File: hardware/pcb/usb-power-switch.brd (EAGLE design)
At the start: 50.8 x 27.9 mm, 15 parts, among them IC1 TPS2024, IC2 LD1117V33

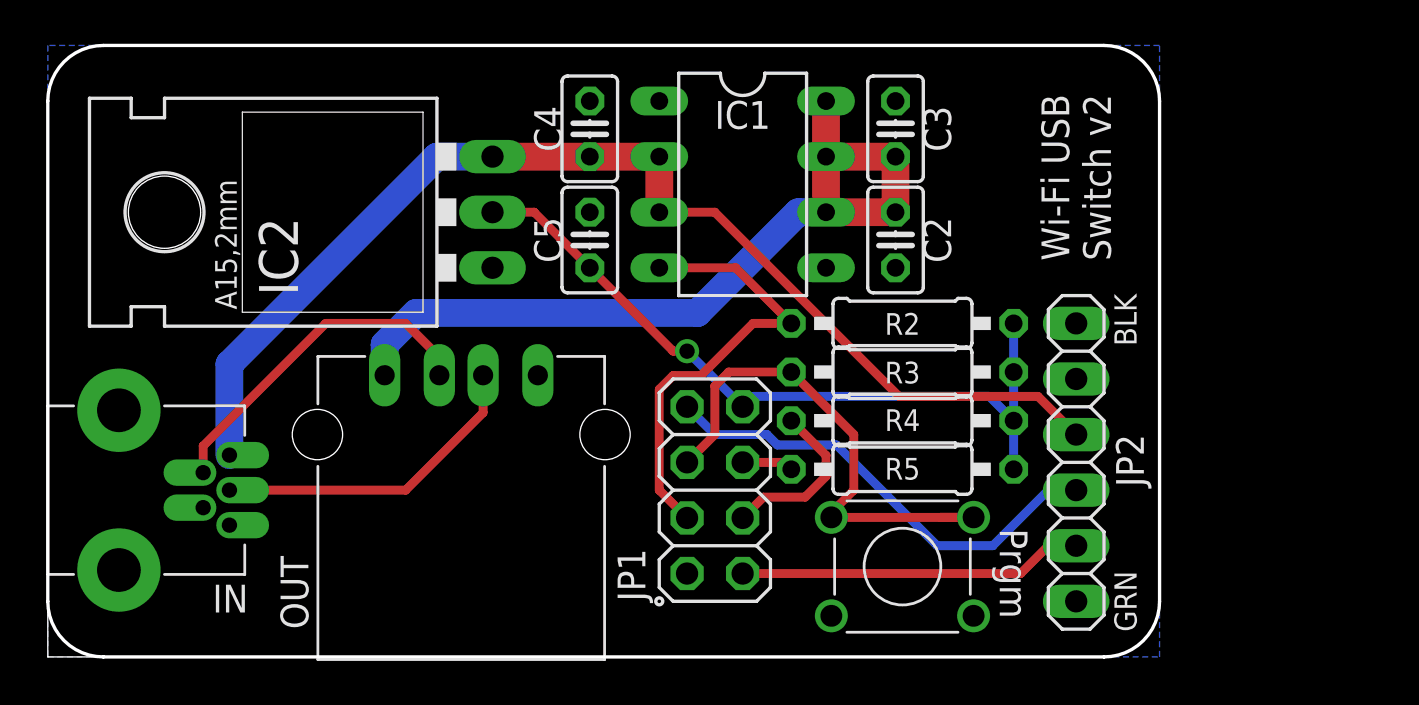
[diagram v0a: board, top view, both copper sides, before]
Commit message: Updated PCB to v3
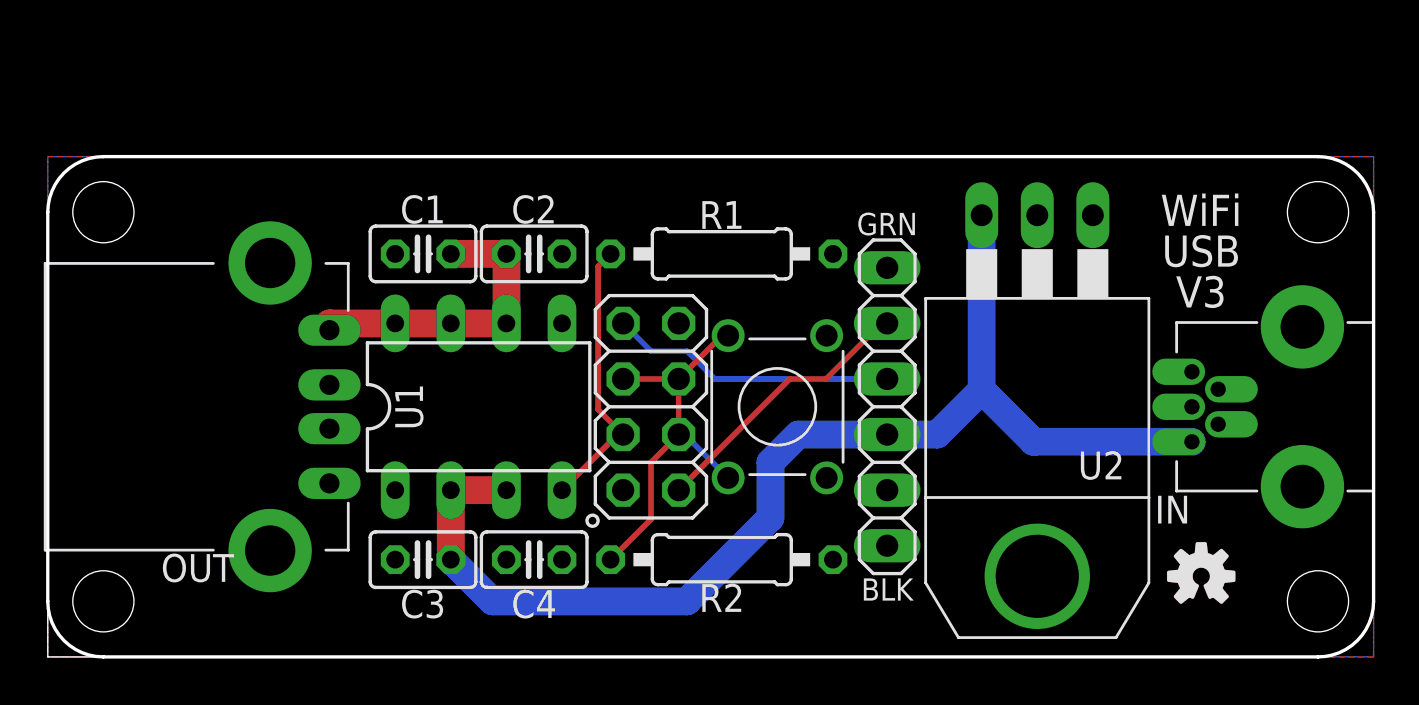
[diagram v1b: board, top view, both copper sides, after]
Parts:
- removed C5: 10uF, rcl:C025-025X050
- removed IC1: TPS2024, ic-package:DIL08
- removed IC2: LD1117V33, SparkFun-PowerIC:78XXL
- removed JP1: ESP-01, pinhead:2X04
- removed JP2: FTDI 3.3V, pinhead:1X06
- removed R3, R4, R5: 10K, rcl:0207/10
- added C1: 22uF, rcl:C025-025X050
- added J1: ESP8266-01, pinhead:2X04
- added J2: FTDI 3.3V, pinhead:1X06
- added R1: 10K, rcl:0207/10
- added U$1: (no value), SparkFun-Aesthetics:OSHW-LOGO-S
- added U$2: (no value), SparkFun-Aesthetics:OSHW-LOGO-S_COPPER
- added U1: TPS2024, ic-package:DIL08
- added U2: LD1117V33, my-custom:TO-220
- C3: value 22uF -> 0.1uF
- C4: value 0.1uF -> 10uF
- IN: value USB-MINI-B -> WM17115-ND
- OUT: value USB-A -> UE27AC54100-ND
- S1: value TACTILE-BUTTON-MJTP1230 -> MJTP1230
- moved IN 57.5 mm to (57.4, 11.4), turned to 90 degrees
- moved C3 29.2 mm to (17.1, 4.45), turned to 180 degrees
- moved C4 19.8 mm to (22.2, 4.45), turned to 180 degrees
- moved C2 16.5 mm to (22.2, 18.4), turned to 0 degrees
- moved R2 13.6 mm to (30.8, 4.45)
- moved S1 9.27 mm to (33.3, 11.4), turned to 90 degrees
- moved OUT 8.82 mm to (10.2, 11.4), turned to 270 degrees
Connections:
- removed net CH_PD: JP1.3, R4.1
- removed net D+: IN.D+, OUT.P$3
- removed net D-: IN.D-, OUT.P$2
- removed net GPIO0: JP1.6, R3.1, S1.P$1, S1.P$3
- removed net RST: JP1.5, R5.1
- new net PU: J1.3, J1.5, J1.6, R2.1, S1.P$1, S1.P$3
- net /EN: now also J1.4, R1.1, U1.4; no longer IC1.4, JP1.4, R2.1
- net DTR: now also J2.6; no longer JP2.6
- net GND: now also C1.2, IN.GND1, IN.GND4, J1.2, J2.1, J2.2, OUT.P$5, OUT.P$6, U1.1, U2.P$1; no longer C3.2, C5.2, IC1.1, IC2.IN, JP1.2, JP2.1, JP2.2
- net RXI: now also J1.8, J2.4; no longer JP1.8, JP2.4
- net TXO: now also J1.1, J2.5; no longer JP1.1, JP2.5
- net VCC: now also C4.1, J1.7, R1.2, U2.P$2, U2.P$4; no longer C5.1, IC2.GND, JP1.7, R3.2, R4.2, R5.2
- net VIN: now also C3.1, J2.3, U1.2, U1.3, U2.P$3; no longer C4.1, IC1.2, IC1.3, IC2.OUT, JP2.3
- net VOUT: now also C1.1, U1.6, U1.7, U1.8; no longer C3.1, IC1.6, IC1.7, IC1.8
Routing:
- net VCC: track 34.8 -> 0.00 mm, vias 1 -> 0
- net GPIO0: track 24.1 -> 0.00 mm
- net VOUT: track 38.1 -> 14.1 mm
- net PU: track 0.00 -> 18.2 mm
- net D-: track 15.8 -> 0.00 mm
- net D+: track 14.8 -> 0.00 mm
- net RXI: track 21.5 -> 13.1 mm
- net /EN: track 20.8 -> 12.8 mm
- net CH_PD: track 7.80 -> 0.00 mm
- net TXO: track 15.8 -> 12.7 mm
- net RST: track 2.35 -> 0.00 mm
- net VIN: track 53.5 -> 54.8 mm
- added copper zone on layer 1, net VCC
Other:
- board size 50.8 x 27.9 mm -> 60.6 x 22.9 mm
- board text added: "WiFi USB V3"
- board text removed: "Prgm"
- board text removed: "Wi-Fi USB Switch v2"
